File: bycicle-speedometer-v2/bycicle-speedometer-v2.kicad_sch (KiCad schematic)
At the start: 2 parts, among them J1 Conn_01x04_Pin

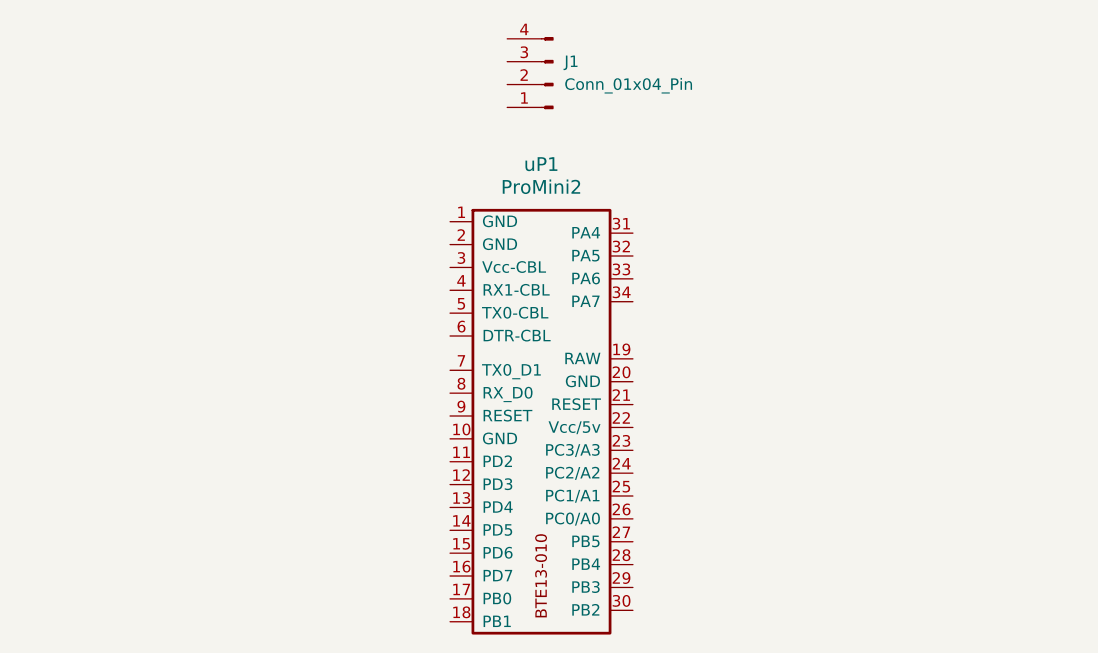
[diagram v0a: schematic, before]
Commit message: initiated schematic update
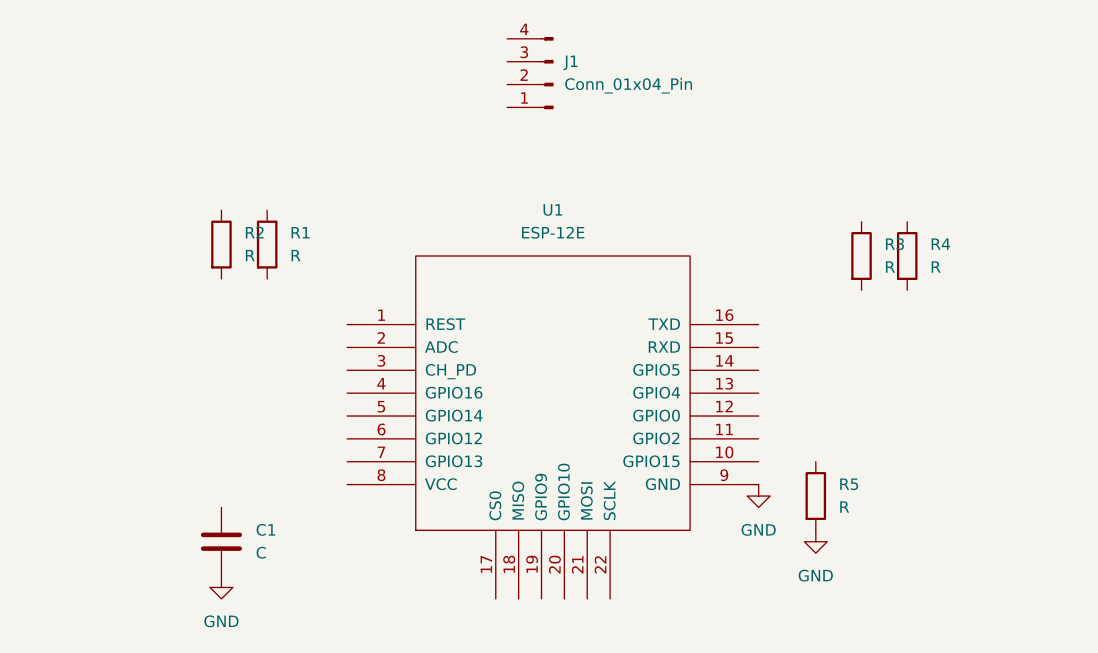
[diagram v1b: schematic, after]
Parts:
- removed uP1: ProMini2, Pro mini:Pro_Mini, symbol j_ProcessorBoards:ProMini2
- added C1: C, symbol Device:C
- added R1, R2, R3, R4, R5: R, symbol Device:R
- added U1: ESP-12E, ESP8266:ESP-12E, symbol ESP8266:ESP-12E
- J1: footprint Display:Adafruit_SSD1306 -> Connector_PinSocket_2.54mm:PinSocket_1x04_P2.54mm_Vertical
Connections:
- new net GND: C1.2, R5.2, U1.9 (GND)

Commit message: modified schematic
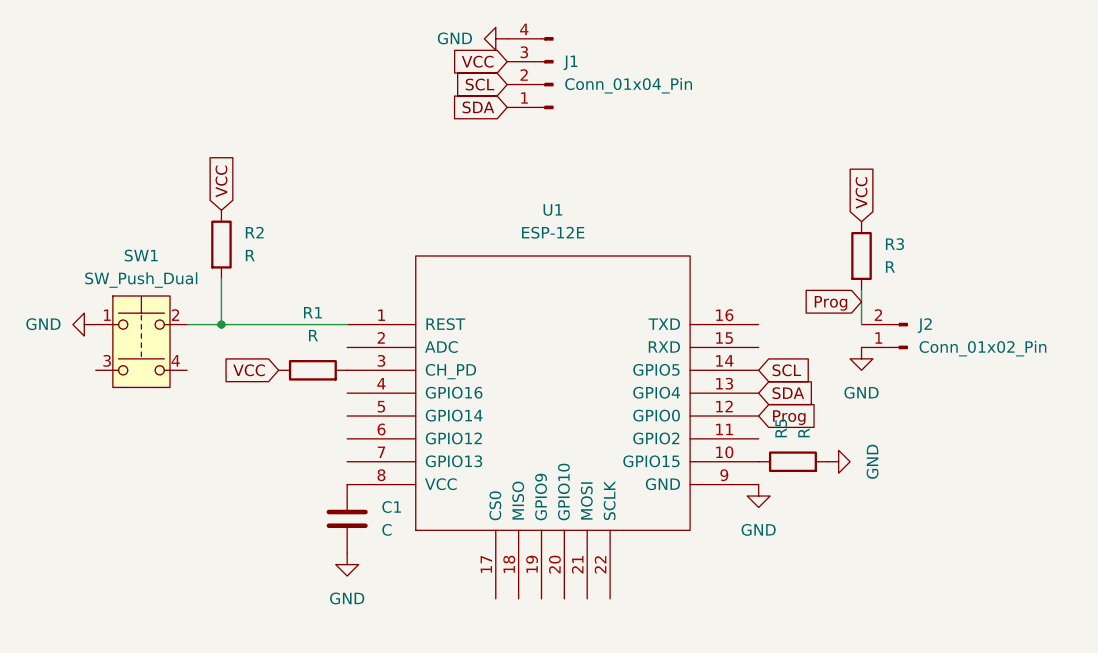
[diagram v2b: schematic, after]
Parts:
- removed R4: R, symbol Device:R
- added J2: Conn_01x02_Pin, symbol Connector:Conn_01x02_Pin
- added SW1: SW_Push_Dual, symbol Switch:SW_Push_Dual
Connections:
- net GND: now also J1.4 (Pin_4), J2.1 (Pin_1), SW1.1
- net at U1.1 (REST): now also R2.2, SW1.2
- net at U1.10 (GPIO15): now also R5.1
- net Prog: now reaches U1.12 (GPIO0)
- net Prog: now also R3.2, J2.2 (Pin_2)
- net SDA: now reaches U1.13 (GPIO4)
- net SDA: now also J1.1 (Pin_1)
- net SCL: now reaches U1.14 (GPIO5)
- net SCL: now also J1.2 (Pin_2)
- net at U1.3 (CH_PD): now also R1.2
- net at U1.8 (VCC): now also C1.1
- net VCC: now reaches R2.1
- net VCC: now also J1.3 (Pin_3), R1.1, R3.1
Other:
- moved on the sheet: C1, R1, R5
